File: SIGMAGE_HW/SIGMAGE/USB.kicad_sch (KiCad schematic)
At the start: 45 parts, among them J1 UJ31CHG2SMTTR, J3 TSW10607GS, U13 ESDR0502NMUTBG, U14 93LC56-I/SN, U9 FT2232HLTRAY

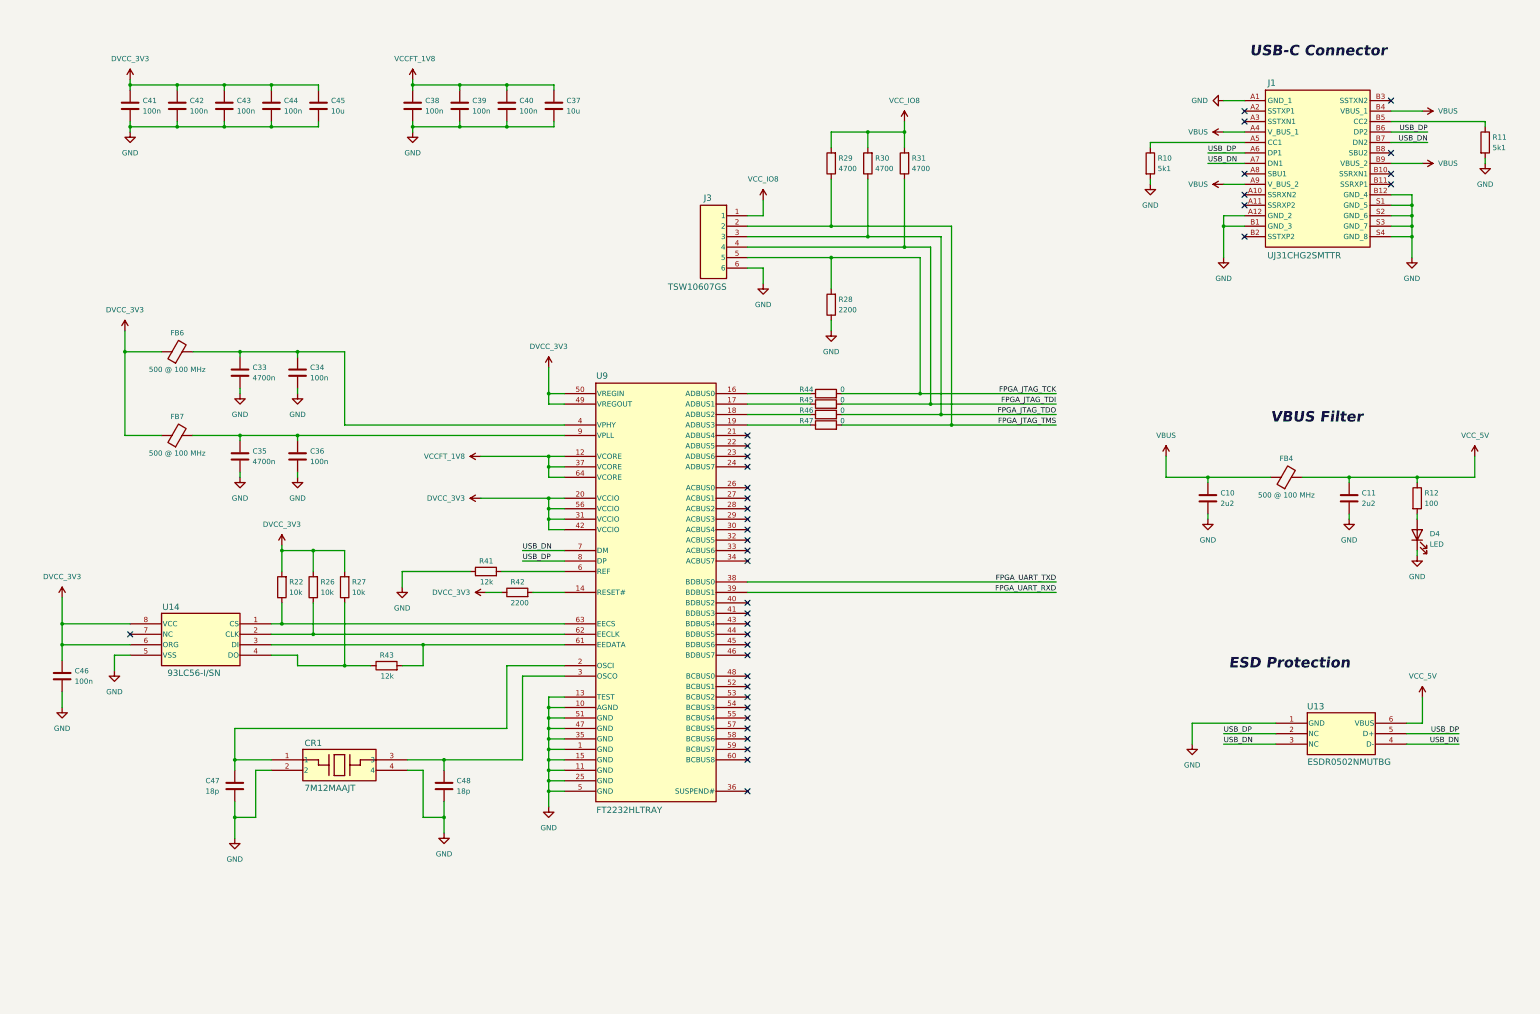
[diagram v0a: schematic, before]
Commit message: changes
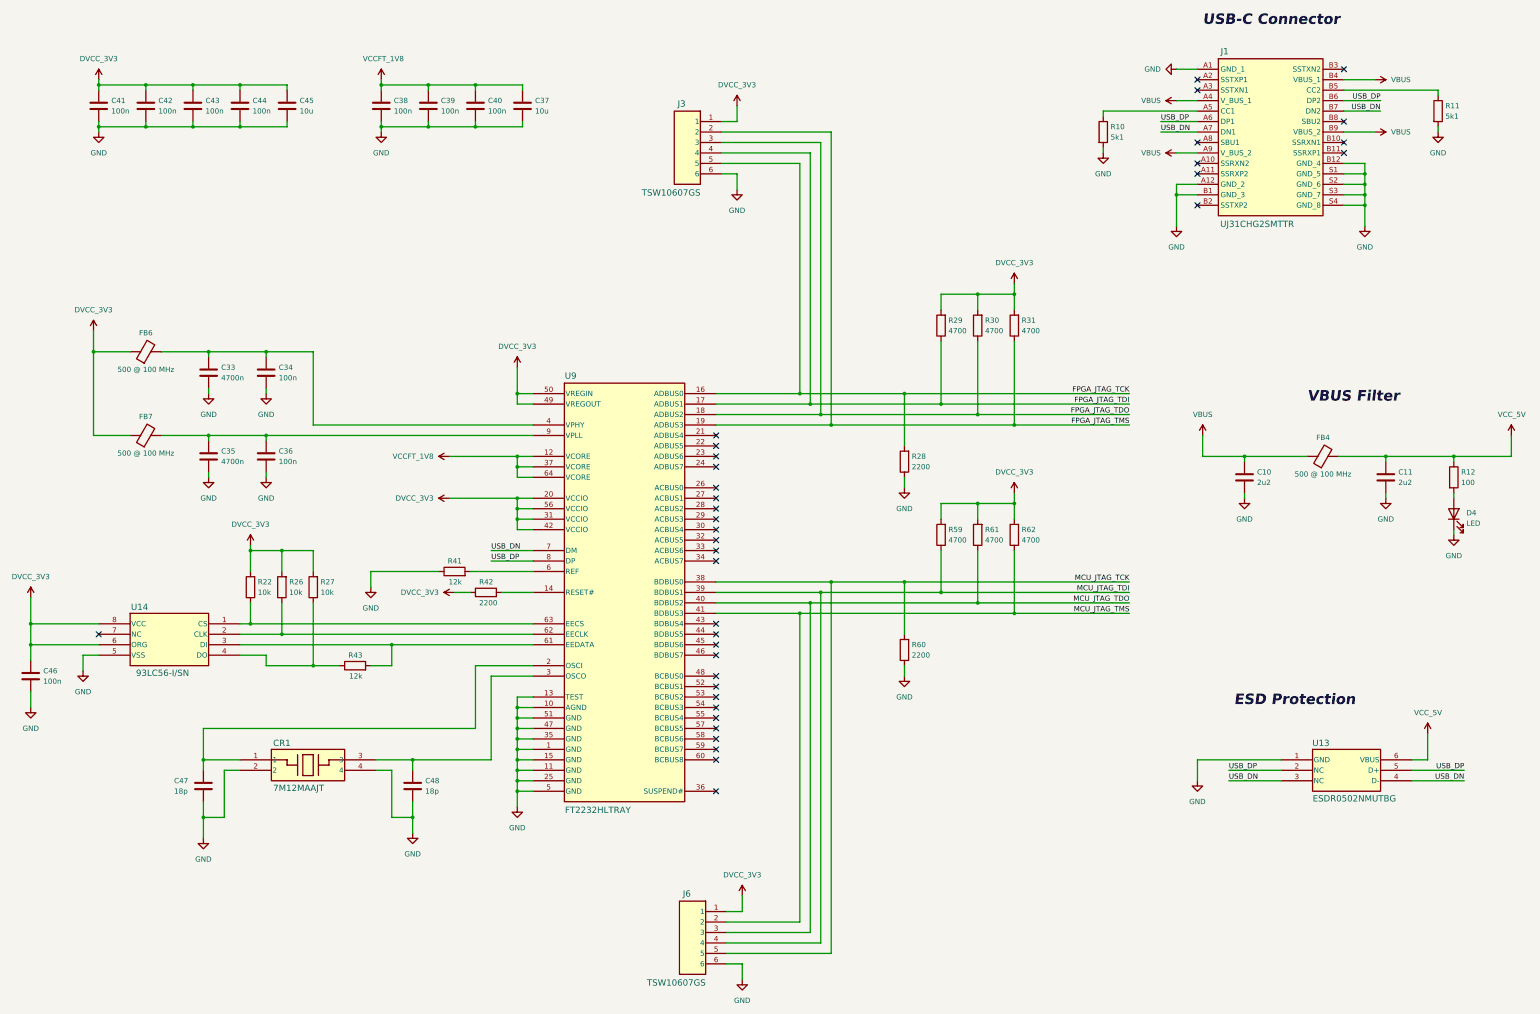
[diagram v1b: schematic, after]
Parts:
- removed R44, R45, R46, R47: 0, Resistor_SMD:R_0603_1608Metric, symbol Device:R
- added J6: TSW10607GS, SIGMAGE:TSW10607GS, symbol SIGMAGE:TSW10607GS
- added R59, R61, R62: 4700, Resistor_SMD:R_0603_1608Metric, symbol Device:R
- added R60: 2200, Resistor_SMD:R_0603_1608Metric, symbol Device:R
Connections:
- net VCC_IO8 is gone; now on net DVCC_3V3: J3.1, R29.2, R30.2, R31.2
- net DVCC_3V3: now also J6.1, R59.2, R61.2, R62.2
- net FPGA_JTAG_TCK: now also U9.16 (ADBUS0)
- net FPGA_JTAG_TDI: now also R29.1, U9.17 (ADBUS1); no longer R31.1
- net FPGA_JTAG_TDO: now also U9.18 (ADBUS2)
- net FPGA_JTAG_TMS: now also R31.1, U9.19 (ADBUS3); no longer R29.1
- net GND: now also J6.6, R60.1
- net MCU_JTAG_TDO: now reaches U9.40 (BDBUS2)
- net MCU_JTAG_TDO: now also J6.3, R61.1
- net MCU_JTAG_TMS: now reaches U9.41 (BDBUS3)
- net MCU_JTAG_TMS: now also J6.2, R62.1
- net FPGA_UART_RXD renamed MCU_JTAG_TDI
- net MCU_JTAG_TDI: now also J6.4, R59.1
- net FPGA_UART_TXD renamed MCU_JTAG_TCK
- net MCU_JTAG_TCK: now also J6.5, R60.2
- no-connect marks 39 -> 37
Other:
- moved on the sheet: C10, C11, C33, C34, C35, C36, C37, C38, C39, C40, C41, C42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
